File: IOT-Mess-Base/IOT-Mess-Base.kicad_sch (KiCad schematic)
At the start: 30 parts, among them J1 Conn_01x09_Pin, J2 TP_4056, Q1 AO3400A, Q2 AO3401A, Q3 AO3400A, Q4 AO3401A, Q5 AO3400A, SW2 SW_Push, SW3 SW_Push, U12 APDS-9960, U13 SHT31-DIS, U17 BH1750FVI-TR, U2 SHT4x, U3 INA219AxDCN, U8 TPL5110

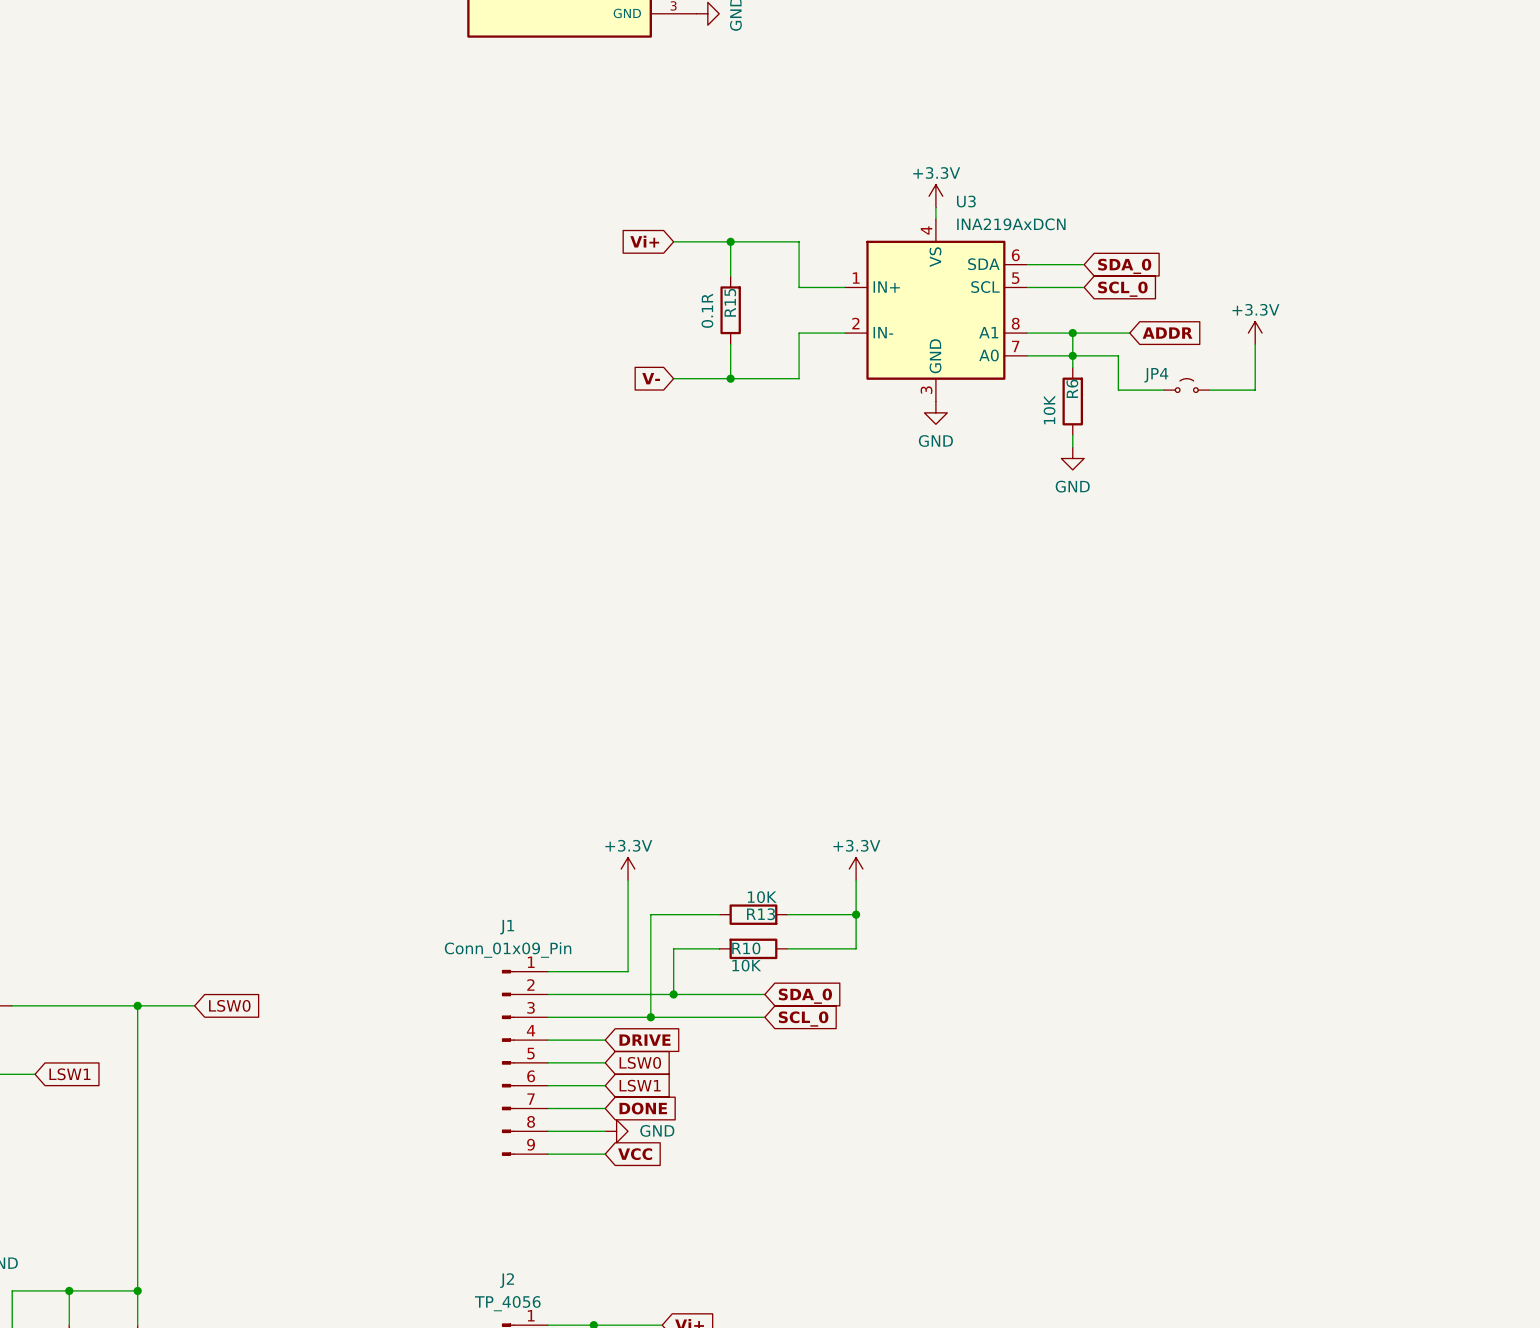
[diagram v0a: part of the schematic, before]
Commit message: did some works.
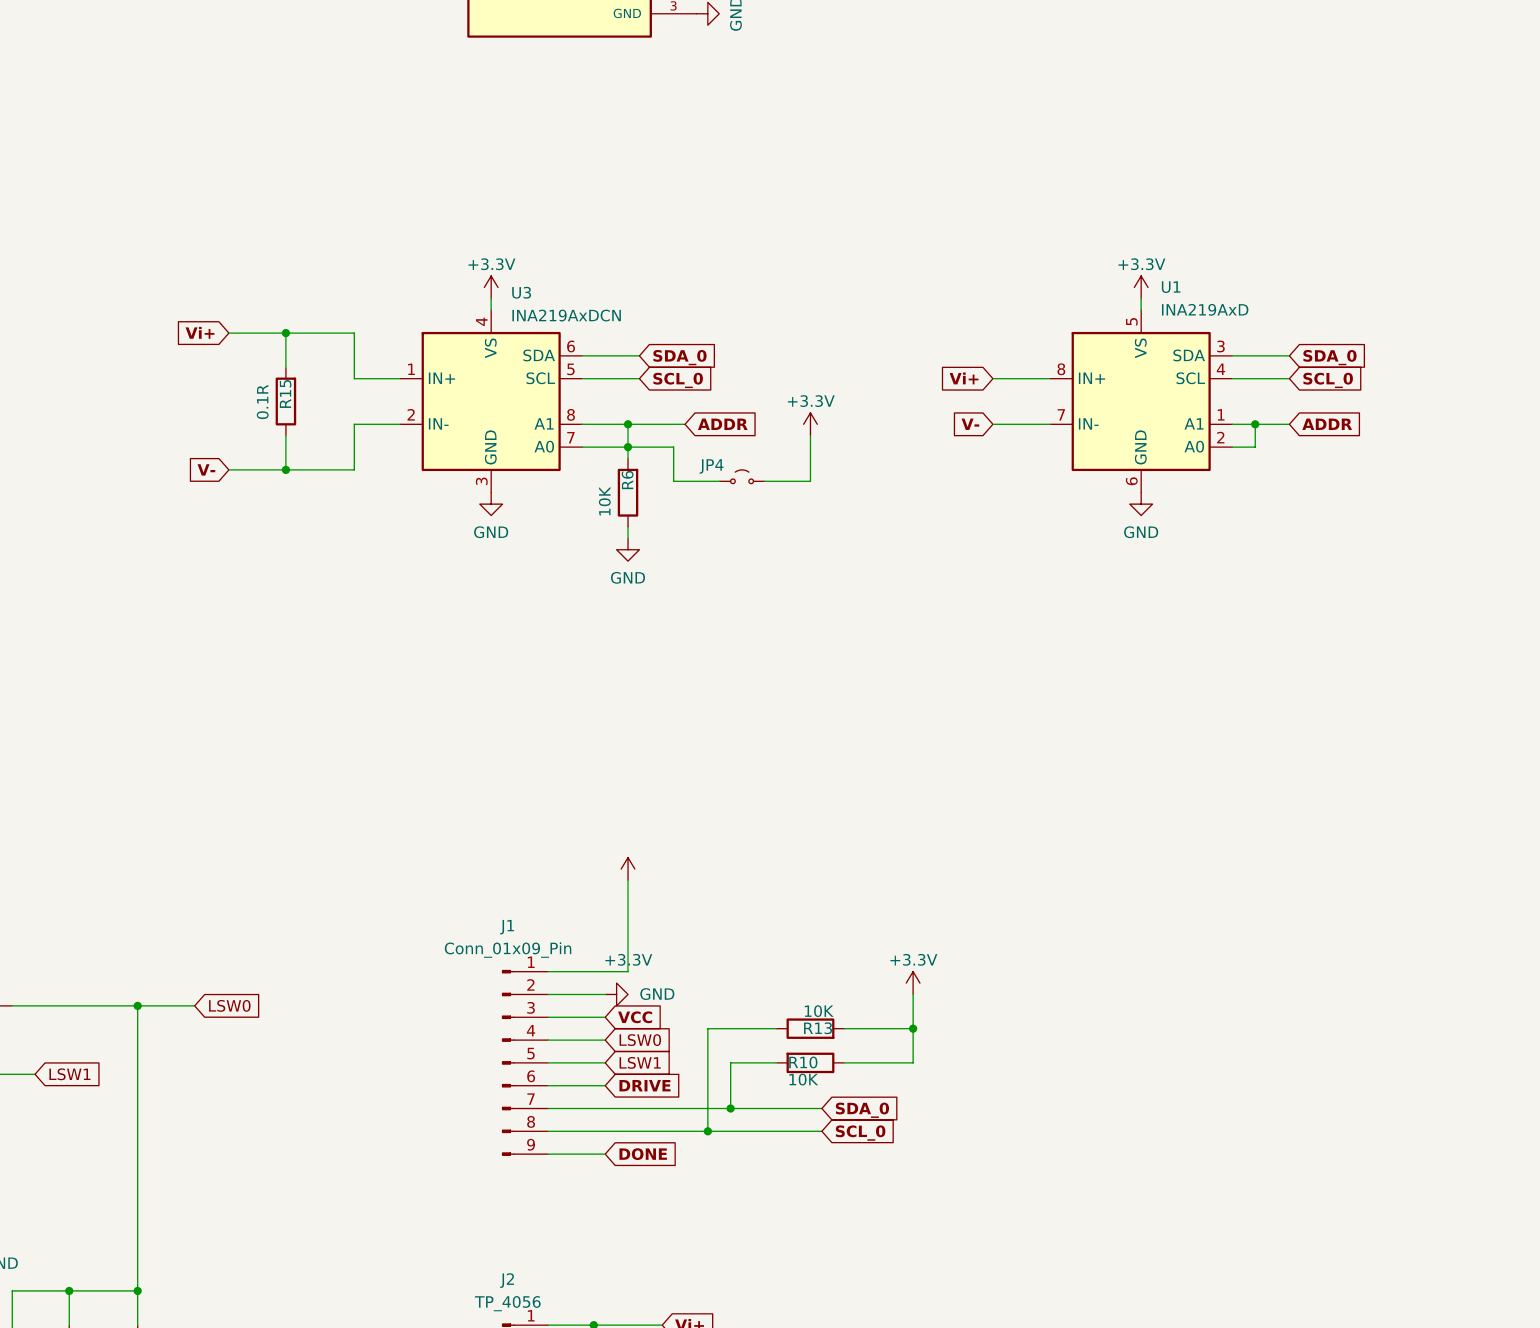
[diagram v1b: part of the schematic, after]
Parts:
- added U1: INA219AxD, Package_SO:SOIC-8_3.9x4.9mm_P1.27mm, symbol Sensor_Energy:INA219AxD
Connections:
- net +3.3V: now also U1.5 (VS)
- net ADDR: now also U1.1 (A1), U1.2 (A0)
- net DONE: now also J1.9 (Pin_9); no longer J1.7 (Pin_7)
- net DRIVE: now also J1.6 (Pin_6); no longer J1.4 (Pin_4)
- net GND: now also J1.2 (Pin_2), U1.6 (GND); no longer J1.8 (Pin_8)
- net LSW0: now also J1.4 (Pin_4); no longer J1.5 (Pin_5)
- net LSW1: now also J1.5 (Pin_5); no longer J1.6 (Pin_6)
- net SCL_0: now also J1.8 (Pin_8), U1.4 (SCL); no longer J1.3 (Pin_3)
- net SDA_0: now also J1.7 (Pin_7), U1.3 (SDA); no longer J1.2 (Pin_2)
- net V-: now also U1.7 (IN-)
- net VCC: now also J1.3 (Pin_3); no longer J1.9 (Pin_9)
- net Vi+: now also U1.8 (IN+)
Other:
- moved on the sheet: JP4, R10, R13, R15, R6, U3
